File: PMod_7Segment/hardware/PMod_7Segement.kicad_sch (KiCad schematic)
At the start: 7 parts, among them J1 Conn_02x06_Odd_Even, U1 GN1640

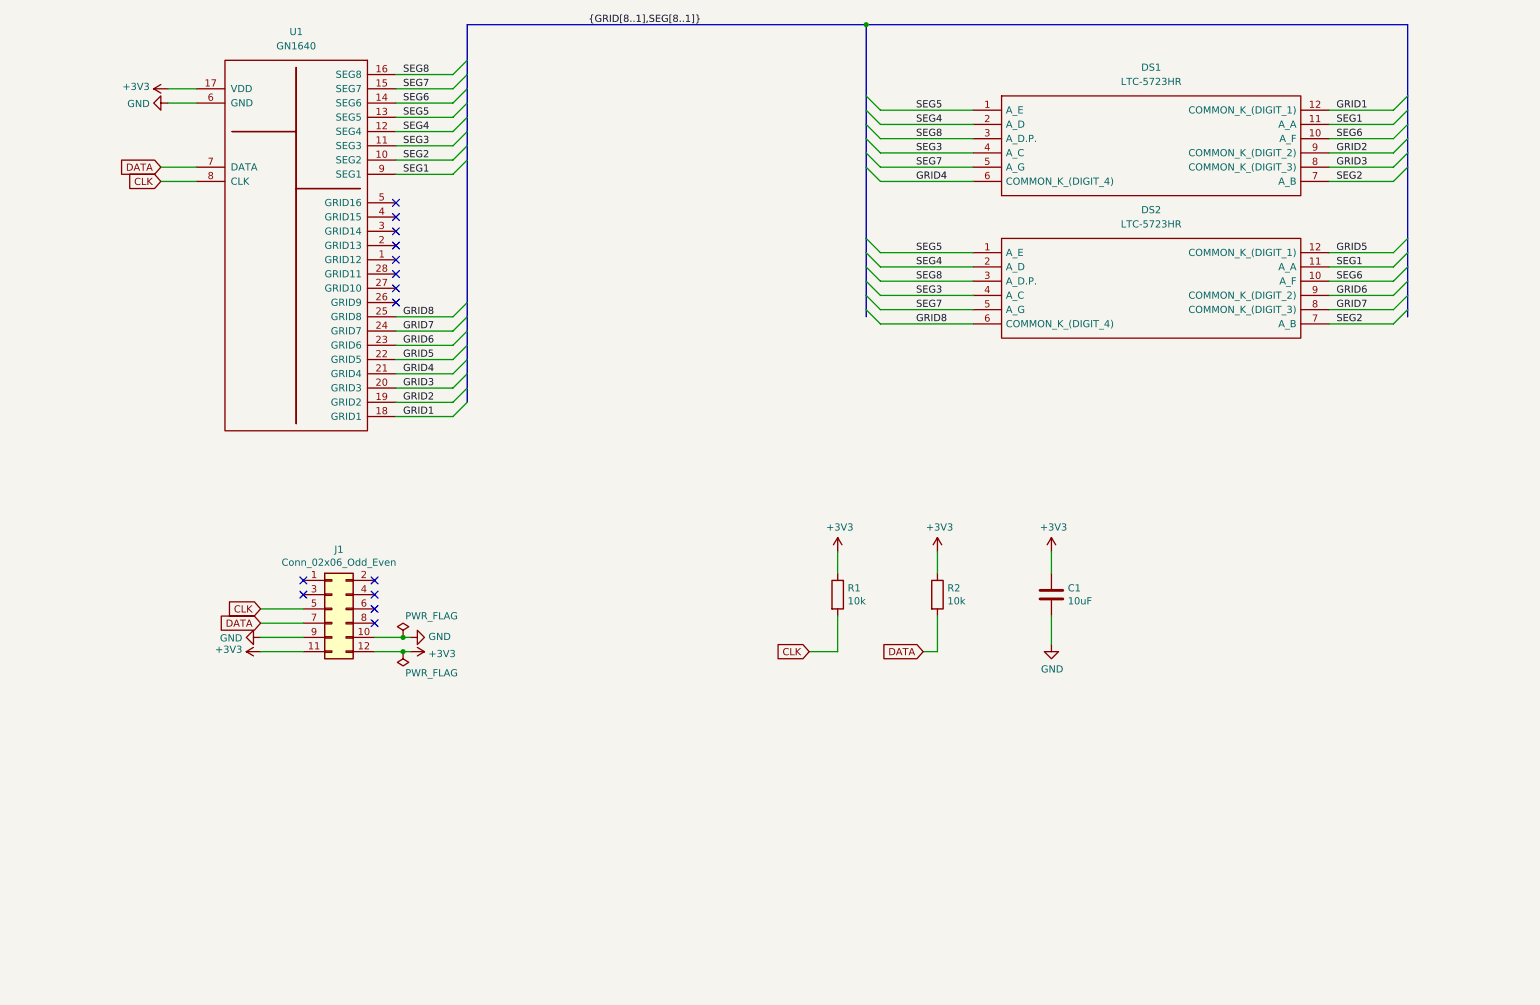
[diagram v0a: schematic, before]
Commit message: Schematic visual improvements and add license
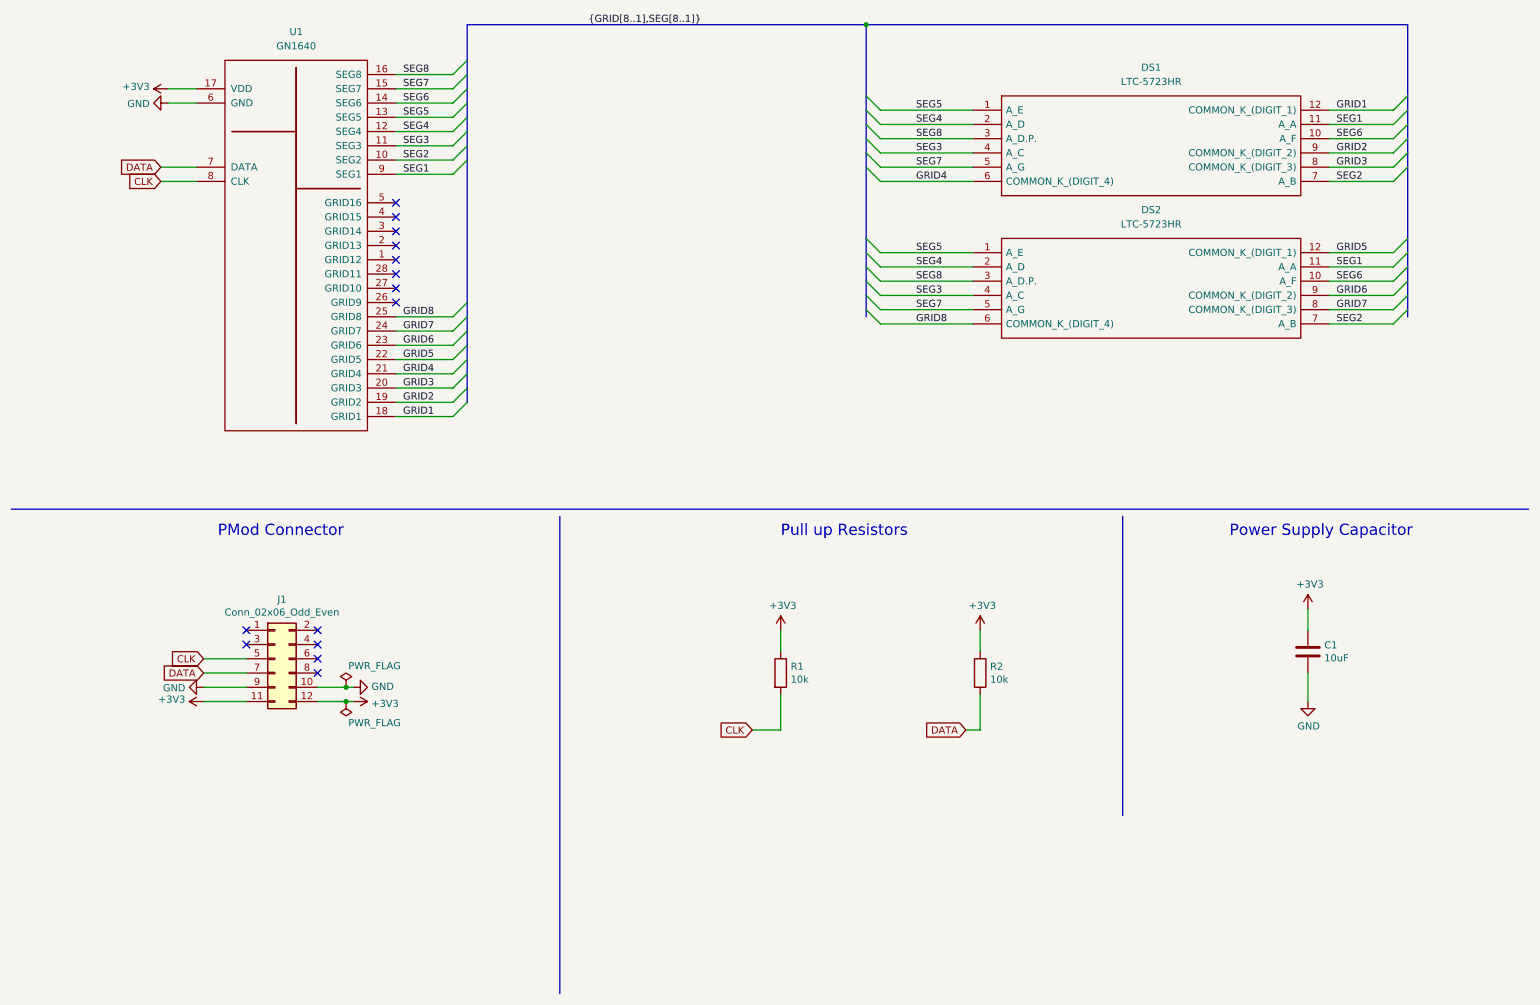
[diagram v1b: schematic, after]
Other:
- note added: "PMod Connector"
- note added: "Power Supply Capacitor"
- note added: "Pull up Resistors"
- company: (none) -> James Horton
- title: (none) -> PMod 7 Segment Display
- moved on the sheet: C1, J1, R1, R2
